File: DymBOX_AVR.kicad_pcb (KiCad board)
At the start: 2 copper layers, 31 parts, among them J2 Conn_01x03_Pin, J3 Conn_01x02_Pin, J4 Conn_01x03_Pin, J5 Conn_02x05_Odd_Even, Q1 BC327, Q2 BC327, Q3 BS170, Q4 BS170, Q5 BC327, U1 ATmega8A-P, U2 CA56-12EWA, U3 L7805, Y1 Crystal

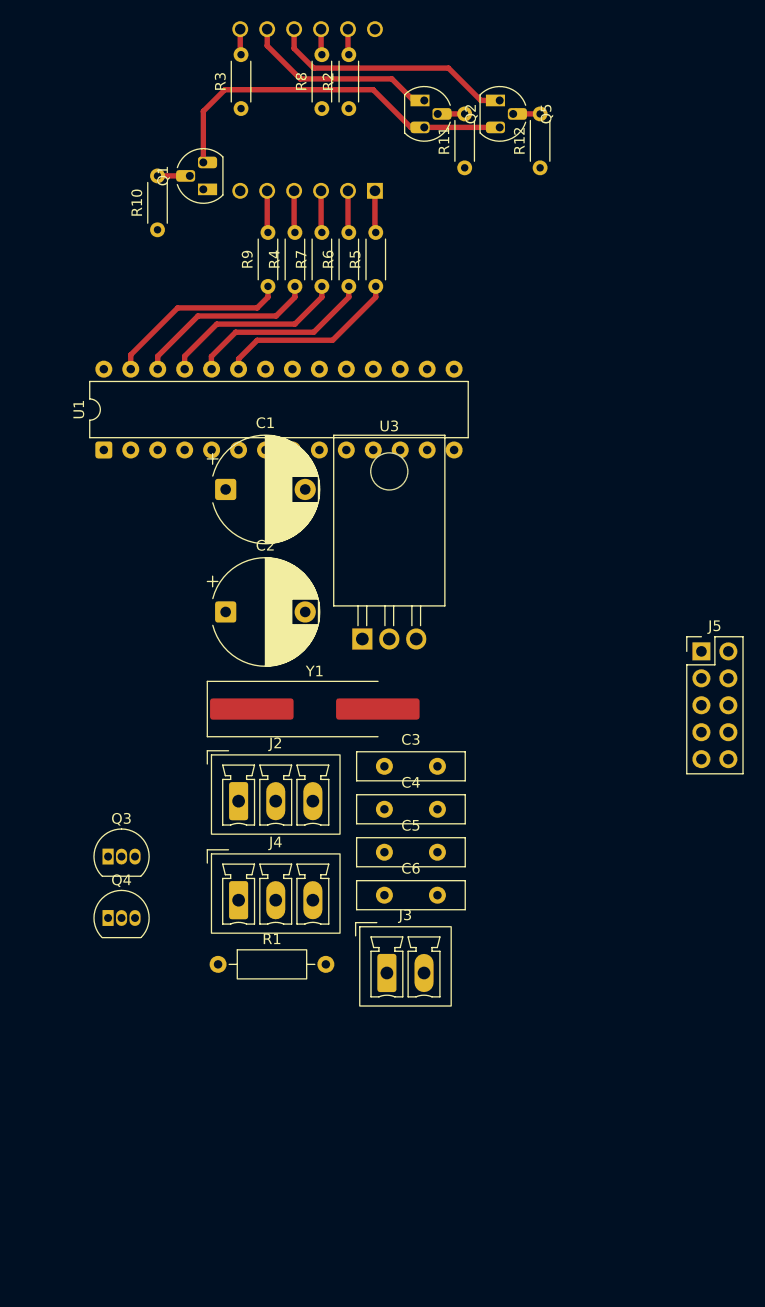
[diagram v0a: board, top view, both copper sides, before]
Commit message: pcb_f
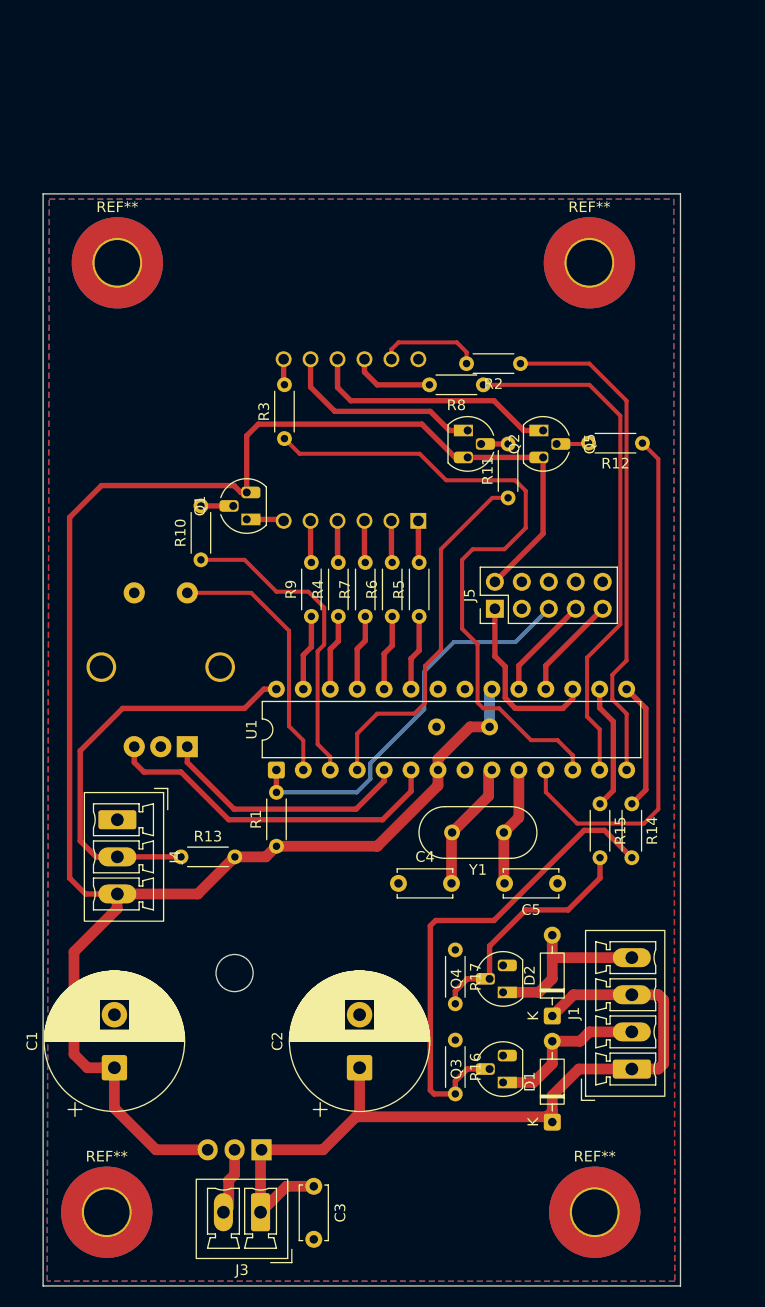
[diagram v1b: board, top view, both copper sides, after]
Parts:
- removed J2: Conn_01x03_Pin, Connector_Phoenix_MC:PhoenixContact_MCV_1,5_3-G-3.5_1x03_P3.50mm_Vertical
- added D1: 1N4148, Diode_THT:D_DO-35_SOD27_P7.62mm_Horizontal, F.Cu at (166.5, 124.5)
- added D2: 1N4148, Diode_THT:D_DO-35_SOD27_P7.62mm_Horizontal, F.Cu at (166.5, 114.5)
- added J1: Conn_01x04_Pin, Connector_Phoenix_MC:PhoenixContact_MCV_1,5_4-G-3.5_1x04_P3.50mm_Vertical, F.Cu at (174.0, 119.5)
- added R13: 4k7, Resistor_THT:R_Axial_DIN0204_L3.6mm_D1.6mm_P5.08mm_Horizontal, F.Cu at (131.5, 99.5)
- added R14: 330, Resistor_THT:R_Axial_DIN0204_L3.6mm_D1.6mm_P5.08mm_Horizontal, F.Cu at (174.0, 94.5)
- added R15: 330, Resistor_THT:R_Axial_DIN0204_L3.6mm_D1.6mm_P5.08mm_Horizontal, F.Cu at (171.0, 94.5)
- added R16: 10k, Resistor_THT:R_Axial_DIN0204_L3.6mm_D1.6mm_P5.08mm_Horizontal, F.Cu at (157.4, 116.8)
- added R17: 10k, Resistor_THT:R_Axial_DIN0204_L3.6mm_D1.6mm_P5.08mm_Horizontal, F.Cu at (157.4, 108.3)
- added REF**: MountingHole_4.3mm_M4_Pad_TopBottom, MountingHole:MountingHole_4.3mm_M4_Pad_TopBottom, F.Cu at (125.5, 43.5)
- added REF**: MountingHole_4.3mm_M4_Pad_TopBottom, MountingHole:MountingHole_4.3mm_M4_Pad_TopBottom, F.Cu at (170.5, 133.0)
- added REF**: MountingHole_4.3mm_M4_Pad_TopBottom, MountingHole:MountingHole_4.3mm_M4_Pad_TopBottom, F.Cu at (124.5, 133.0)
- added REF**: MountingHole_4.3mm_M4_Pad_TopBottom, MountingHole:MountingHole_4.3mm_M4_Pad_TopBottom, F.Cu at (170.0, 43.5)
- added SW1: RotaryEncoder_Switch, Rotary_Encoder:RotaryEncoder_Alps_EC12E-Switch_Vertical_H20mm_CircularMountingHoles, B.Cu at (132.1, 89.1)
- C1, C2: footprint Capacitor_THT:CP_Radial_D10.0mm_P7.50mm -> Capacitor_THT:CP_Radial_D13.0mm_P5.00mm
- C3, C4, C5: footprint Capacitor_THT:C_Disc_D10.0mm_W2.5mm_P5.00mm -> Capacitor_THT:C_Disc_D5.0mm_W2.5mm_P5.00mm
- C6: footprint Capacitor_THT:C_Disc_D10.0mm_W2.5mm_P5.00mm -> Capacitor_THT:C_Disc_D5.0mm_W2.5mm_P5.00mm; moved to B.Cu
- J4: value Conn_01x03_Pin -> DS18B20
- Q1: footprint Package_TO_SOT_THT:TO-92L_HandSolder -> Package_TO_SOT_THT:TO-92_HandSolder
- Q3, Q4: footprint Package_TO_SOT_THT:TO-92_Inline -> Package_TO_SOT_THT:TO-92_HandSolder
- R1: footprint Resistor_THT:R_Axial_DIN0207_L6.3mm_D2.5mm_P10.16mm_Horizontal -> Resistor_THT:R_Axial_DIN0204_L3.6mm_D1.6mm_P5.08mm_Horizontal
- R10, R11, R12: value R -> 1k
- U3: footprint Package_TO_SOT_THT:TO-220F-3_Horizontal_TabDown -> Package_TO_SOT_THT:TO-220-3_Horizontal_TabDown; moved to B.Cu
- Y1: footprint Crystal:Crystal_SMD_HC49-SD_HandSoldering -> Crystal:Crystal_HC49-U_Vertical
- moved C1 55.5 mm to (125.2, 119.4), turned to 90 degrees
- moved U3 49.1 mm to (139.1, 127.1), turned to 180 degrees
- moved C2 44.8 mm to (148.3, 119.4), turned to 90 degrees
- moved Q3 42.9 mm to (161.9, 120.8), turned to 90 degrees
- moved C3 40.1 mm to (144.0, 130.6), turned to -90 degrees
- moved Q4 37.9 mm to (161.9, 112.3), turned to 90 degrees
- moved U1 34.3 mm to (140.5, 91.3)
- moved R11 31.4 mm to (162.3, 65.7)
- moved Q2 31.4 mm to (158.5, 59.3)
- moved R3 31.4 mm to (141.3, 60.1)
- moved Q1 31.4 mm to (137.7, 67.7)
- moved R10 31.4 mm to (133.4, 71.5)
- moved R6 31.4 mm to (151.4, 76.8)
- moved R7 31.4 mm to (148.9, 76.8)
- moved R9 31.4 mm to (143.8, 76.8)
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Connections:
- J4 pad 1: unconnected-(J4-Pin_1-Pad1) -> GND
- J4 pad 2: unconnected-(J4-Pin_2-Pad2) -> Net-(J4-Pin_2)
- J4 pad 3: GND -> +5V
- J5 pad 1: unconnected-(J5-Pin_1-Pad1) -> /MOSI
- J5 pad 3: unconnected-(J5-Pin_3-Pad3) -> GND
- J5 pad 7: unconnected-(J5-Pin_7-Pad7) -> /SCK
- J5 pad 8: unconnected-(J5-Pin_8-Pad8) -> GND
- J5 pad 9: unconnected-(J5-Pin_9-Pad9) -> /MISO
- Q3 pad 1: unconnected-(Q3-D-Pad1) -> Net-(D1-A)
- Q3 pad 2: unconnected-(Q3-G-Pad2) -> Net-(Q3-G)
- Q3 pad 3: unconnected-(Q3-S-Pad3) -> GND
- Q4 pad 1: unconnected-(Q4-D-Pad1) -> Net-(D2-A)
- Q4 pad 2: unconnected-(Q4-G-Pad2) -> Net-(Q4-G)
- Q4 pad 3: unconnected-(Q4-S-Pad3) -> GND
- U1 pad 11: unconnected-(U1-PD5-Pad11) -> /DIG_2
- U1 pad 15: unconnected-(U1-PB1-Pad15) -> Net-(U1-PB1)
- U1 pad 16: unconnected-(U1-PB2-Pad16) -> Net-(U1-PB2)
- U1 pad 17: unconnected-(U1-PB3-Pad17) -> /MOSI
- U1 pad 18: unconnected-(U1-PB4-Pad18) -> /MISO
- U1 pad 19: unconnected-(U1-PB5-Pad19) -> /SCK
- U1 pad 2: /DIG_0 -> /BTN
- U1 pad 28: unconnected-(U1-PC5-Pad28) -> Net-(J4-Pin_2)
- U1 pad 3: /DIG_1 -> /DIG_0
- U1 pad 4: /DIG_2 -> /DIG_1
- U1 pad 5: unconnected-(U1-PD3-Pad5) -> /CLK
- U1 pad 6: unconnected-(U1-PD4-Pad6) -> /DT
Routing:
- net +5V: track 35.4 -> 188.1 mm
- net +12V: track 0.00 -> 77.3 mm
- net /SEG_B: track 0.00 -> 62.0 mm
- net /DIG_2: track 0.00 -> 49.6 mm
- net /SEG_F: track 0.00 -> 49.3 mm
- net /SEG_A: track 0.00 -> 47.4 mm
- net Net-(Q3-G): track 0.00 -> 46.7 mm
- net Net-(J4-Pin_2): track 0.00 -> 39.5 mm
- net /RESET: track 0.00 -> 37.9 mm
- net /DIG_1: track 0.00 -> 34.5 mm
- net /DT: track 0.00 -> 32.9 mm
- net /DIG_0: track 0.00 -> 29.5 mm
- net /BTN: track 0.00 -> 24.8 mm
- net /CLK: track 0.00 -> 24.0 mm
- net Net-(Q4-G): track 0.00 -> 23.0 mm
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- added copper zone on B.Cu, net GND
- added copper zone on F.Cu, net GND
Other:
- board outline added: 60.1 x 102.9 mm

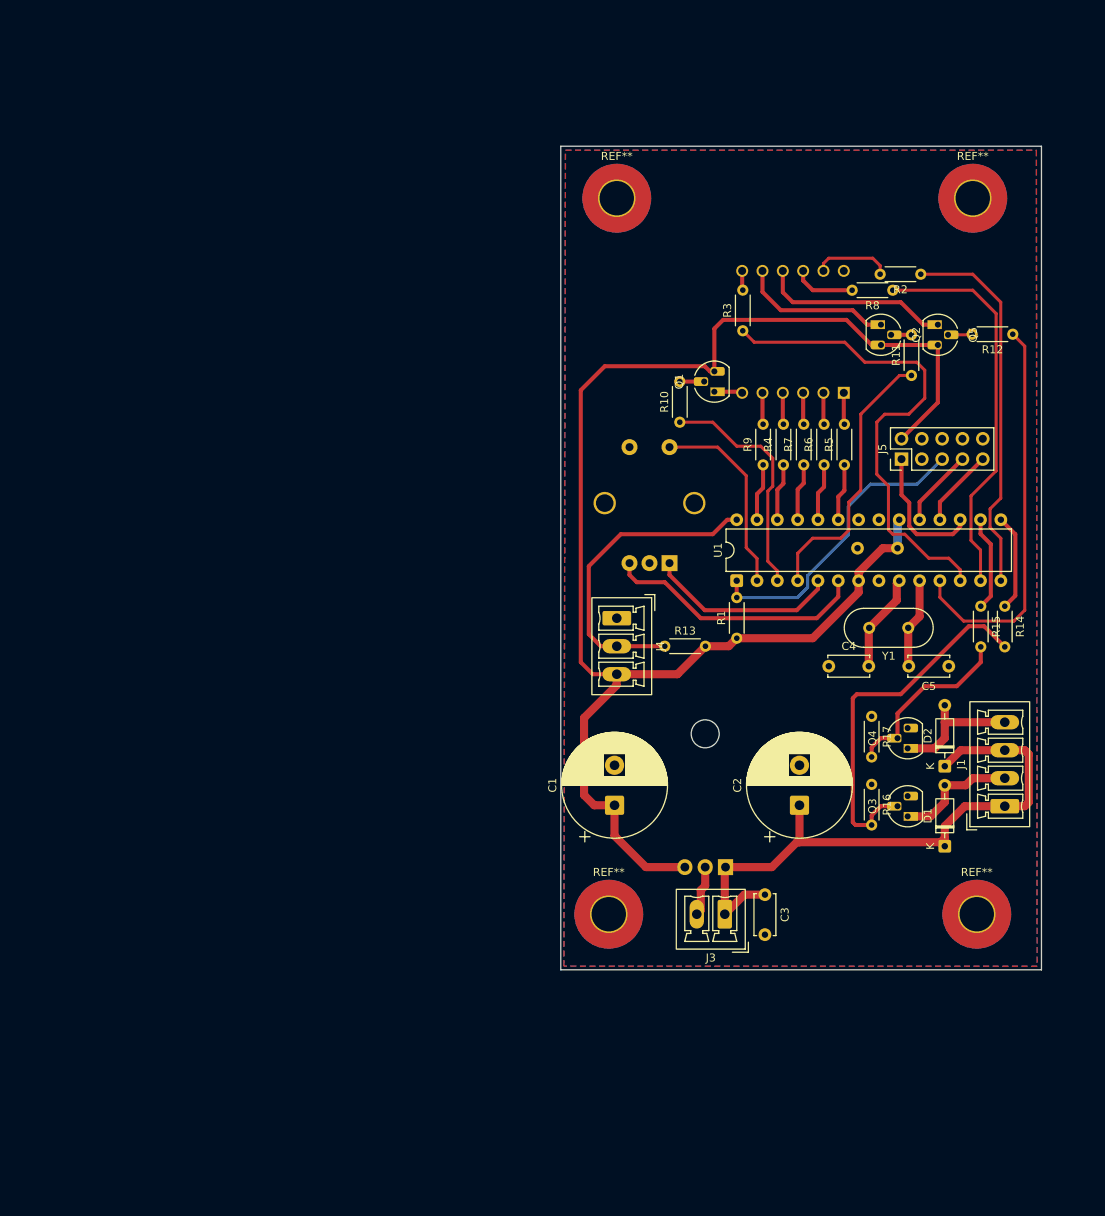
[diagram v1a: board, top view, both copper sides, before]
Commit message: pcb_transfo
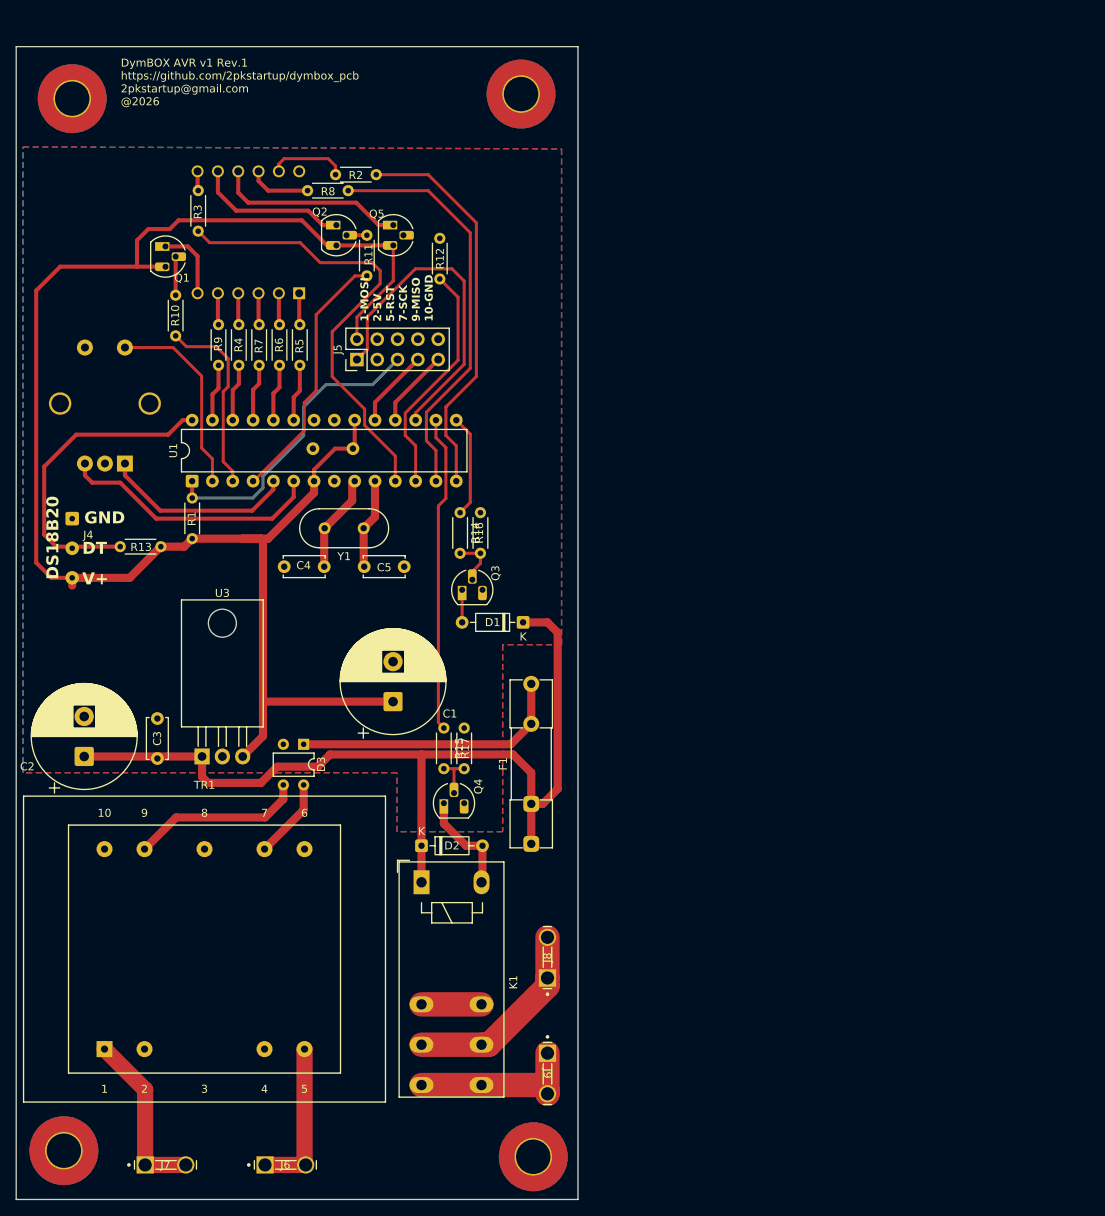
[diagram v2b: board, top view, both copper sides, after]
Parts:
- removed J1: Conn_01x04_Pin, Connector_Phoenix_MC:PhoenixContact_MCV_1,5_4-G-3.5_1x04_P3.50mm_Vertical
- removed J3: Conn_01x02_Pin, Connector_Phoenix_MC:PhoenixContact_MCV_1,5_2-G-3.5_1x02_P3.50mm_Vertical
- added D3: D_Bridge_+-AA, Diode_THT:Diode_Bridge_DIP-4_W5.08mm_P2.54mm, F.Cu at (86.4, 111.8)
- added F1: Fuse, Fuse:Fuseholder_Clip-5x20mm_Littelfuse_111_Inline_P20.00x5.00mm_D1.05mm_Horizontal, F.Cu at (114.8, 124.2)
- added J6: Conn_01x01_Pin, 2pkstartup:TRM2_62409-1_TEC, F.Cu at (86.6, 164.3)
- added J7: Conn_01x01_Pin, 2pkstartup:TRM2_62409-1_TEC, F.Cu at (71.6, 164.3)
- added J8: Conn_01x01_Pin, 2pkstartup:TRM2_62409-1_TEC, F.Cu at (116.8, 135.9)
- added J9: Conn_01x01_Pin, 2pkstartup:TRM2_62409-1_TEC, F.Cu at (116.8, 155.4)
- added K1: RT314A24, Relay_THT:Relay_SPDT_Schrack-RT1-16A-FormC_RM5mm, F.Cu at (101.1, 129.0)
- added TR1: TEZ6.0-D-1, Transformer_THT:Transformer_Breve_TEZ-38x45, F.Cu at (61.5, 149.9)
- C5: value C_Small -> Q1
- J4: footprint Connector_Phoenix_MC:PhoenixContact_MCV_1,5_3-G-3.5_1x03_P3.50mm_Vertical -> Connector_Wire:SolderWire-0.127sqmm_1x03_P3.7mm_D0.48mm_OD1mm
- R1: value R -> 10k
- U3: moved to F.Cu
- Y1: value Crystal -> 16MHz
- moved C2 89.6 mm to (58.9, 113.3)
- moved C3 77.8 mm to (68.1, 113.5), turned to 90 degrees
- moved REF** 74.2 mm to (56.4, 162.6)
- moved R12 72.0 mm to (103.4, 53.6), turned to 90 degrees
- moved Q1 71.0 mm to (69.1, 49.5), turned to -90 degrees
- moved C6 69.2 mm to (92.5, 74.8)
- moved J5 69.2 mm to (93.0, 63.7)
- moved R7 69.2 mm to (80.8, 64.4)
- moved SW1 69.2 mm to (64.0, 76.7)
- moved C4 69.2 mm to (83.9, 89.6)
- moved C5 69.2 mm to (98.9, 89.6)
- moved J4 69.2 mm to (57.4, 83.6)
- moved Q2 69.2 mm to (90.5, 46.9)
- moved Q5 69.2 mm to (97.6, 46.9)
- moved R1 69.2 mm to (72.4, 86.1)
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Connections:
- U1 pad 11: /DIG_2 -> /SEG_B
- U1 pad 12: /SEG_B -> /DIG_2
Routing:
- net Net-(Q3-G): track 46.7 -> 6.26 mm
- net +12V: track 77.3 -> 114.8 mm
- net Net-(D3-+): track 0.00 -> 34.5 mm
- net Net-(U1-PB2): track 11.9 -> 39.7 mm
- net Net-(J8-Pin_1): track 0.00 -> 24.9 mm
- net /MOSI: track 16.9 -> 41.1 mm
- net Net-(D3-Pad3): track 0.00 -> 21.7 mm
- net Net-(J7-Pin_1): track 0.00 -> 21.7 mm
- net Net-(J9-Pin_1): track 0.00 -> 21.5 mm
- net /DIG_2: track 49.6 -> 29.5 mm
- net Net-(J6-Pin_1): track 0.00 -> 19.6 mm
- net Net-(Q4-G): track 23.0 -> 5.59 mm
- net +5V: track 188.1 -> 203.0 mm
- net Net-(D1-A): track 15.4 -> 4.06 mm
- net Net-(D3-Pad4): track 0.00 -> 10.0 mm
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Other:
- board size 60.1 x 102.9 mm -> 70.2 x 144.1 mm
- board text added: "1-MOSI 2-5V 5-RST 7-SCK 9-MISO 10-GND"
- board text added: "DS18B20"
- board text added: "DT"
- board text added: "DymBOX AVR v1 Rev.1 https://github.com/2pkstartup/dymbox_pcb 2pkstartup@gmail.com @2026"
- board text added: "GND"
- board text added: "V+"
